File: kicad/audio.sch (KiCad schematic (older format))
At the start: 50 parts, among them J401 KATE_3.5MM_6, J402 KATE_3.5MM_6, J403 KATE_3.5MM_6, U401 AD824

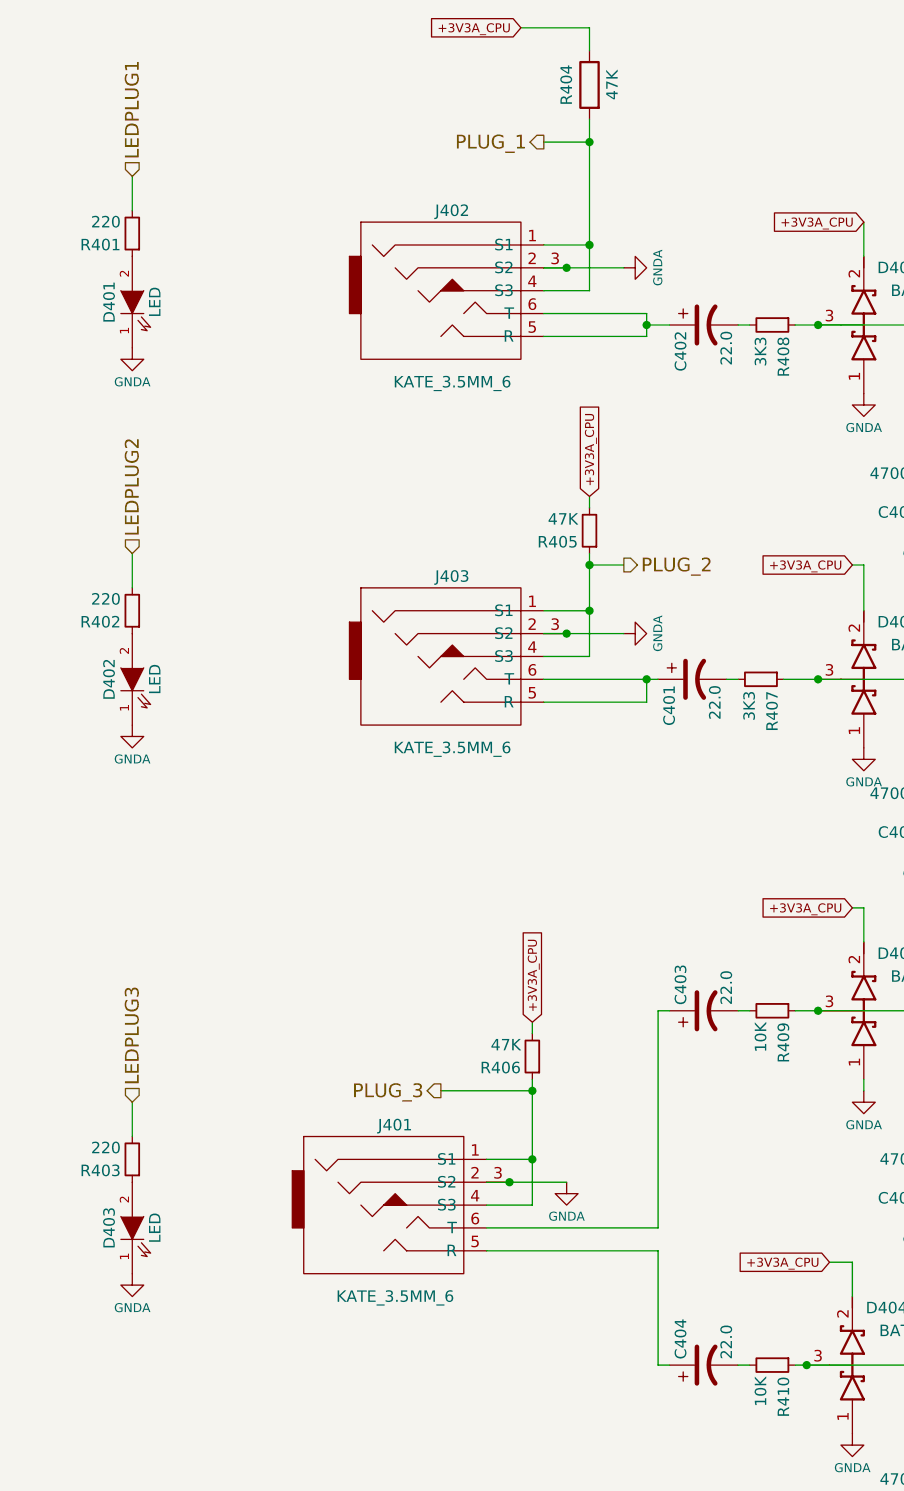
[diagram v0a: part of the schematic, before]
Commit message: before moving headphone amp to the left
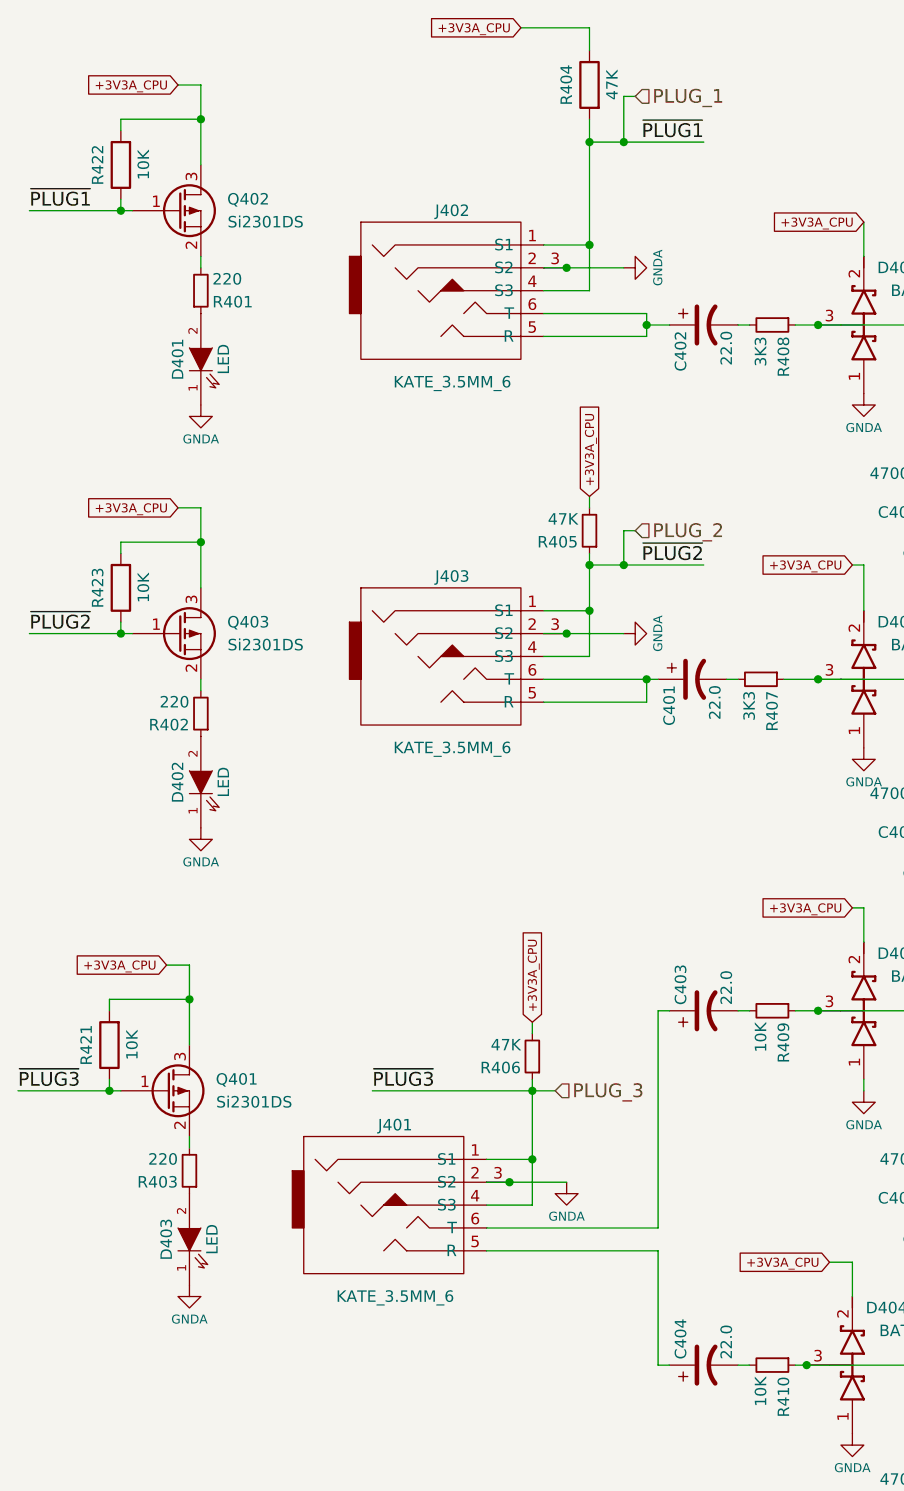
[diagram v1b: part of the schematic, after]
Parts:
- added Q401, Q402, Q403: Si2301DS, TO_SOT_Packages_SMD:SOT-23, symbol Q_PMOS_GSD
- added R421, R422, R423: 10K, Resistors_SMD:R_0805, symbol R
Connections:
- net +3V3A_CPU: now also Q401.3 (D), Q402.3 (D), Q403.3 (D), R421.2, R422.2, R423.2
- net PLUG_1: now also Q402.1 (G), R422.1
- net PLUG_2: now also Q403.1 (G), R423.1
- net PLUG_3: now also Q401.1 (G), R421.1
- net LEDPLUG1: no longer names the net of R401.2
- net LEDPLUG1: now also Q402.2 (S)
- net LEDPLUG2: no longer names the net of R402.2
- net LEDPLUG2: now also Q403.2 (S)
- net LEDPLUG3: no longer names the net of R403.2
- net LEDPLUG3: now also Q401.2 (S)
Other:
- moved on the sheet: D401, D402, D403, R401, R402, R403
